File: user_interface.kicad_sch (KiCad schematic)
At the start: 33 parts, among them J3 Внутр. коннектор потенциометр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, J4 Внутр. коннектор галлетника (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, SW1 Кнопка тактовая 6x6 без фикса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, SW2 Кнопка тактовая 6x6 без фикса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, SW3 Кнопка тактовая 6x6 без фикса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, SW4 Кнопка тактовая 6x6 без фикса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, SW5 Кнопка тактовая 6x6 без фикса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, SW6 Кнопка тактовая 6x6 без фикса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

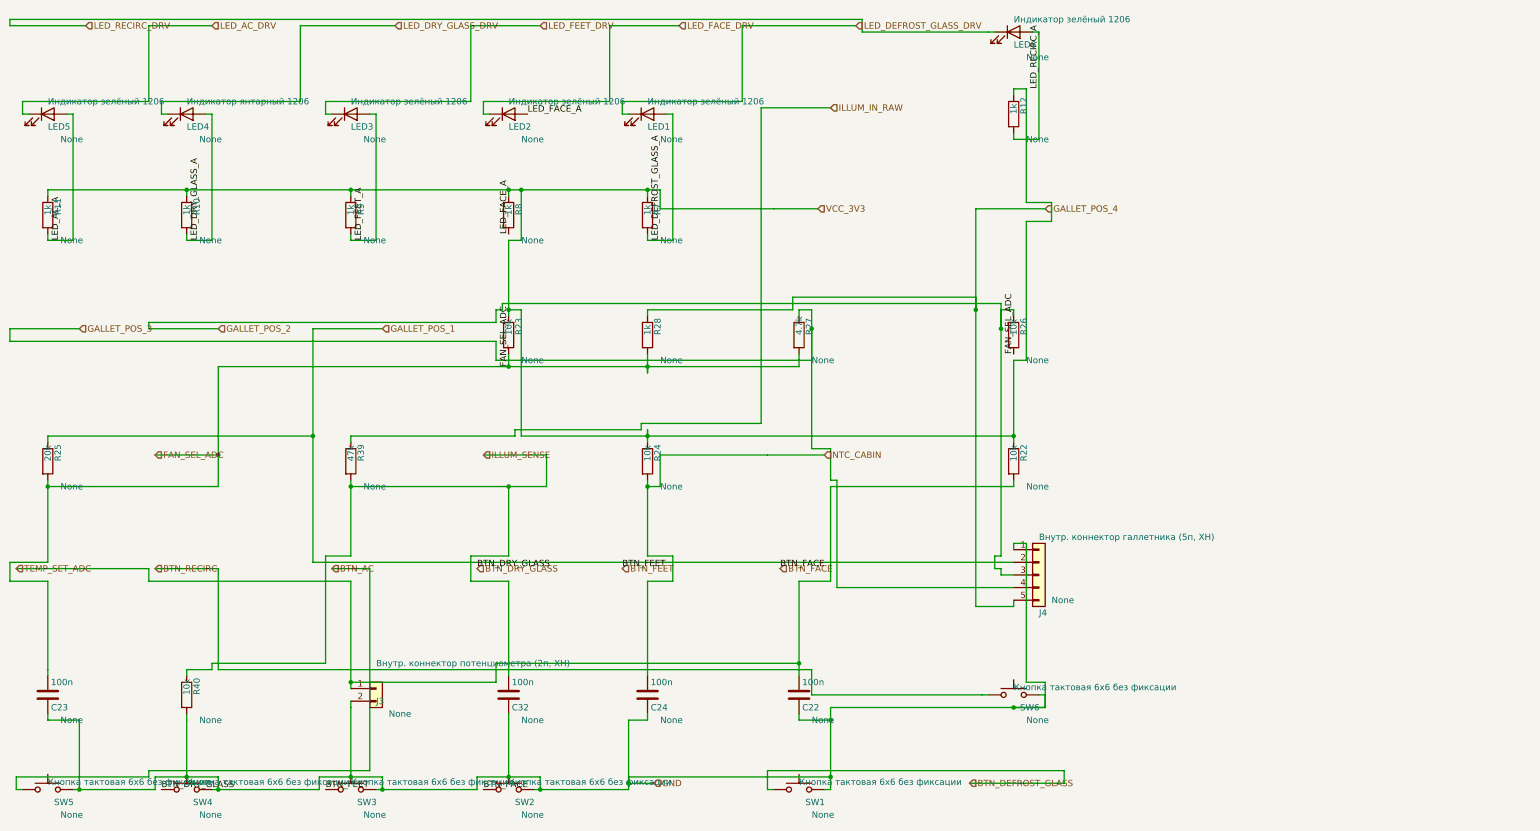
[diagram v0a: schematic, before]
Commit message: tests_fix
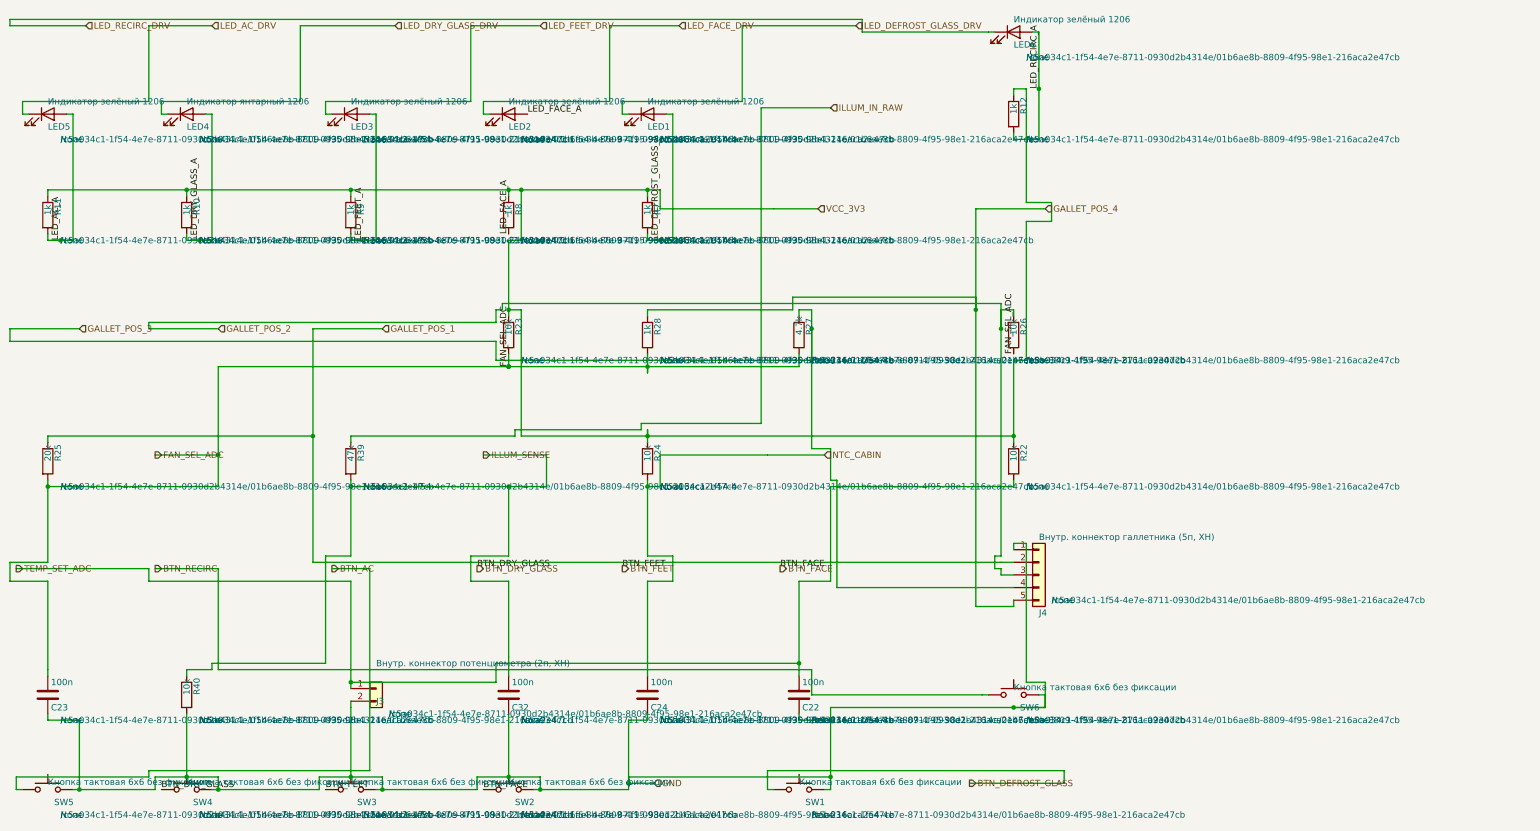
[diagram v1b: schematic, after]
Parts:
- C22, C23, C24, C32, J3, J4, LED1, LED2, LED3, LED4, LED5, LED6, R10, R11, R12, R22, R23, R24, R25, R26, R27, R28, R39, R40, R7, R8, R9, SW1, SW2, SW3, SW4, SW5, SW6: hierarchy_path (none) -> /c5a034c1-1f54-4e7e-8711-0930d2b4314e/01b6ae8b-8809-4f95-98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
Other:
- title: (none) -> climate_control_niva_travel

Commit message: refactoring
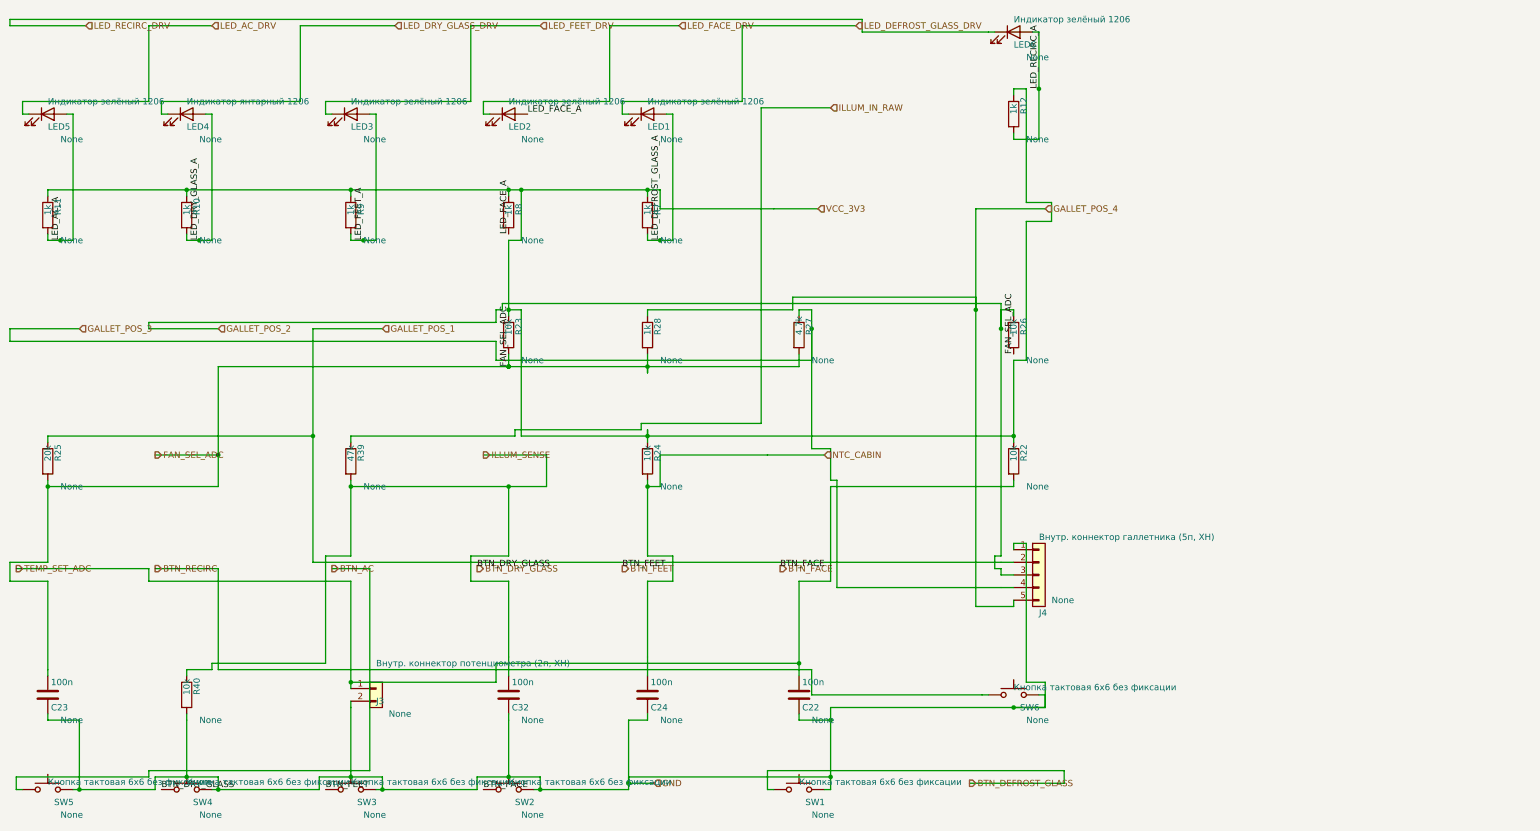
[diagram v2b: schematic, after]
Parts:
- C22, C23, C24, C32, J3, J4, LED1, LED2, LED3, LED4, LED5, LED6, R10, R11, R12, R22, R23, R24, R25, R26, R27, R28, R39, R40, R7, R8, R9, SW1, SW2, SW3, SW4, SW5, SW6: hierarchy_path /c5a034c1-1f54-4e7e-8711-0930d2b4314e/01b6ae8b-8809-4f95-98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 -> (none)

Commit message: refactoring
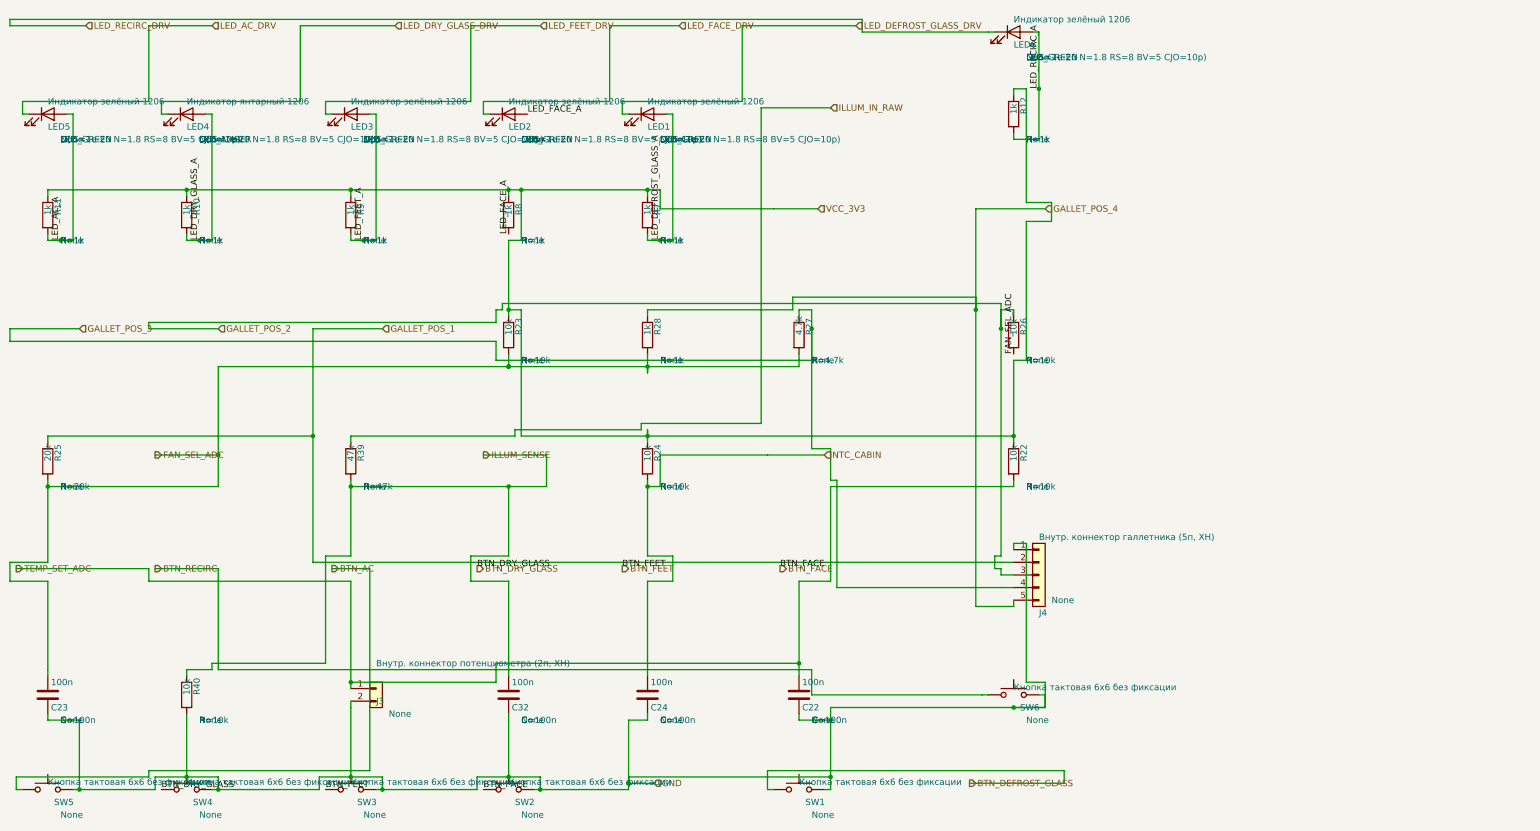
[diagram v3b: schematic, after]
